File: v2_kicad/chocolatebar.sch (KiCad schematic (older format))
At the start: 155 parts, among them J1 Conn_01x04, SW1 SW_Push, U1 ATmega32U4-AU, Y1 Crystal_GND24_Small

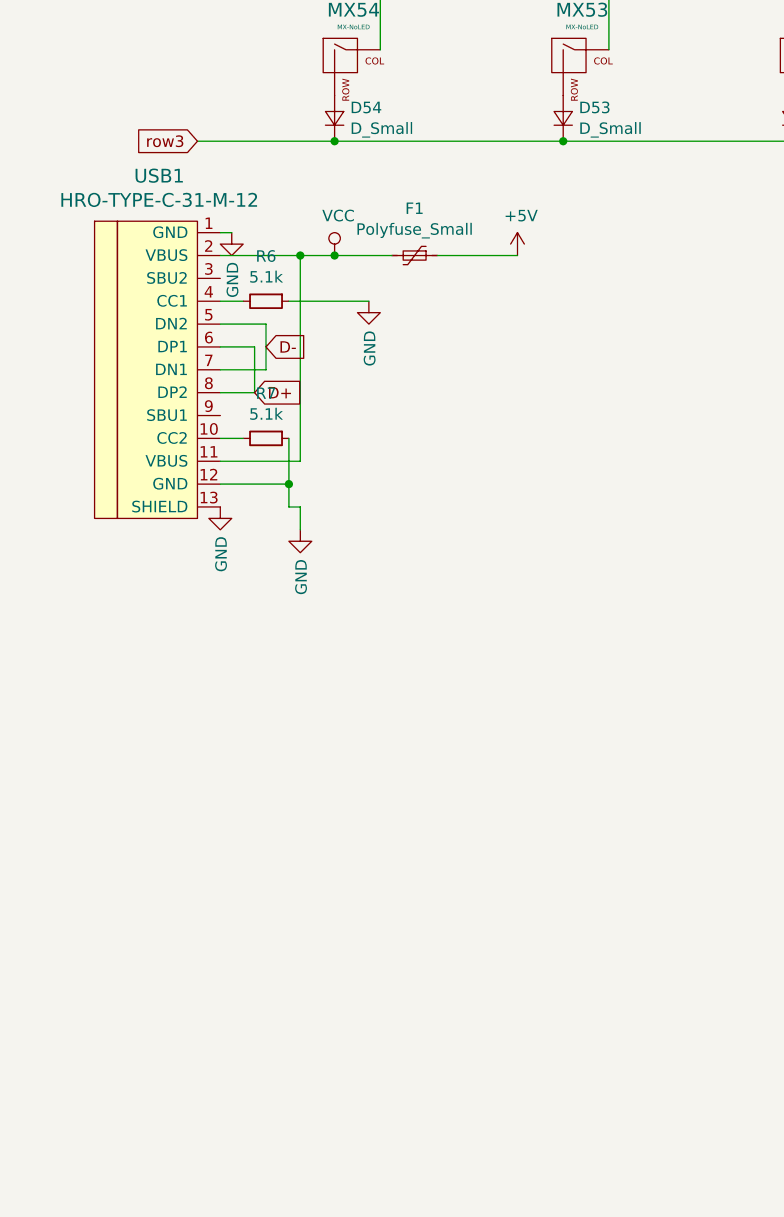
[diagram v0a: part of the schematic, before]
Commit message: V2 update
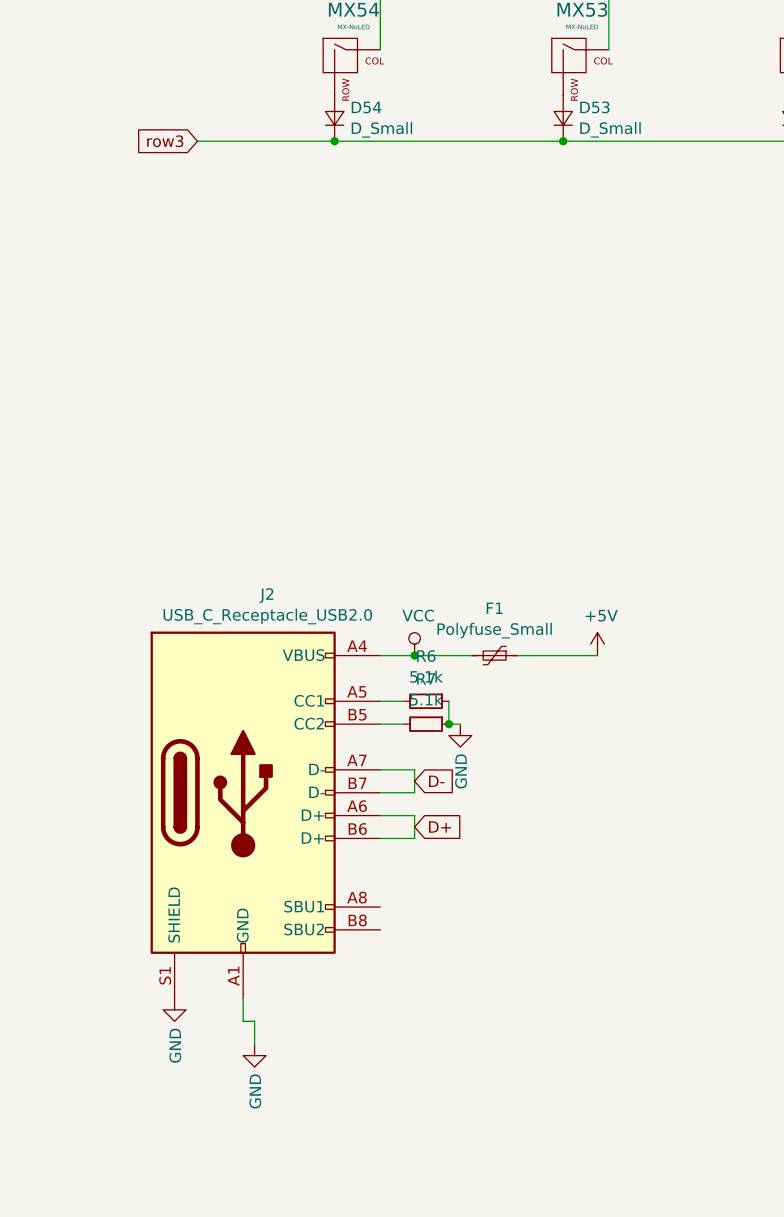
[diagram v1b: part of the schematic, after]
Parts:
- removed USB1: HRO-TYPE-C-31-M-12, Type-C:HRO-TYPE-C-31-M-12-HandSoldering, symbol Type-C:HRO-TYPE-C-31-M-12
- added J2: USB_C_Receptacle_USB2.0, Modified Footprints:USB_C_Receptacle_HRO_TYPE-C-31-M-12, symbol Connector:USB_C_Receptacle_USB2.0
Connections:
- net D+: now also J2.A6 (D+), J2.B6 (D+)
- net D-: now also J2.A7 (D-), J2.B7 (D-)
- net GND: now also J2.A1 (GND), J2.A12 (GND), J2.B1 (GND), J2.B12 (GND), J2.S1 (SHIELD)
- net VCC: now also J2.A4 (VBUS), J2.A9 (VBUS), J2.B4 (VBUS), J2.B9 (VBUS)
- net at R7.2: now also J2.B5 (CC2)
- net at R6.2: now also J2.A5 (CC1)
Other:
- moved on the sheet: F1, R6, R7
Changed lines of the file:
@@
 L Device:Polyfuse_Small F1
 U 1 1 5F2624EF
-P 1950 4900
-F 0 "F1" V 1745 4900 50  0000 C CNN
-F 1 "Polyfuse_Small" V 1836 4900 50  0000 C CNN
-F 2 "Fuse:Fuse_1206_3216Metric" H 2000 4700 50  0001 L CNN
-F 3 "~" H 1950 4900 50  0001 C CNN
-	1    1950 4900
+P 2300 6650
+F 0 "F1" V 2095 6650 50  0000 C CNN
+F 1 "Polyfuse_Small" V 2186 6650 50  0000 C CNN
+F 2 "Fuse:Fuse_1206_3216Metric" H 2350 6450 50  0001 L CNN
+F 3 "~" H 2300 6650 50  0001 C CNN
+	1    2300 6650
 	0    1    1    0
 $EndComp
@@
 L power:+5V #PWR011
 U 1 1 5F26C945
-P 2400 4900
-F 0 "#PWR011" H 2400 4750 50  0001 C CNN
-F 1 "+5V" H 2415 5073 50  0000 C CNN
-F 2 "" H 2400 4900 50  0001 C CNN
-F 3 "" H 2400 4900 50  0001 C CNN
-	1    2400 4900
+P 2750 6650
+F 0 "#PWR011" H 2750 6500 50  0001 C CNN
+F 1 "+5V" H 2765 6823 50  0000 C CNN
+F 2 "" H 2750 6650 50  0001 C CNN
+F 3 "" H 2750 6650 50  0001 C CNN
+	1    2750 6650
 	1    0    0    -1
 $EndComp
@@
 L power:VCC #PWR02
 U 1 1 5F26E1DC
-P 1600 4900
-F 0 "#PWR02" H 1600 4750 50  0001 C CNN
-F 1 "VCC" H 1617 5073 50  0000 C CNN
-F 2 "" H 1600 4900 50  0001 C CNN
-F 3 "" H 1600 4900 50  0001 C CNN
-	1    1600 4900
-	1    0    0    -1
-$EndComp
-Connection ~ 1600 4900
-Wire Wire Line
-	1600 4900 1850 4900
-Wire Wire Line
-	2050 4900 2400 4900
-Text GLabel 1250 5500 2    50   Input ~ 0
+P 1950 6650
+F 0 "#PWR02" H 1950 6500 50  0001 C CNN
+F 1 "VCC" H 1967 6823 50  0000 C CNN
+F 2 "" H 1950 6650 50  0001 C CNN
+F 3 "" H 1950 6650 50  0001 C CNN
+	1    1950 6650
+	1    0    0    -1
+$EndComp
+Connection ~ 1950 6650
+Wire Wire Line
+	1950 6650 2200 6650
+Wire Wire Line
+	2400 6650 2750 6650
+Text GLabel 1950 7400 2    50   Input ~ 0
 D+
-Text GLabel 1300 5300 2    50   Input ~ 0
+Text GLabel 1950 7200 2    50   Input ~ 0
 D-
-$Comp
-L power:GND #PWR01
-U 1 1 5F2AB771
-P 1150 4800
-F 0 "#PWR01" H 1150 4550 50  0001 C CNN
-F 1 "GND" V 1155 4672 50  0000 R CNN
-F 2 "" H 1150 4800 50  0001 C CNN
-F 3 "" H 1150 4800 50  0001 C CNN
-	1    1150 4800
-	1    0    0    -1
-$EndComp
-$Comp
-L Type-C:HRO-TYPE-C-31-M-12 USB1
-U 1 1 5F08F542
-P 1000 5350
-F 0 "USB1" H 833 6147 60  0000 C CNN
-F 1 "HRO-TYPE-C-31-M-12" H 833 6041 60  0000 C CNN
-F 2 "Type-C:HRO-TYPE-C-31-M-12-HandSoldering" H 1000 5350 60  0001 C CNN
-F 3 "" H 1000 5350 60  0001 C CNN
-	1    1000 5350
-	1    0    0    -1
-$EndComp
 Text GLabel 11400 5350 0    50   Input ~ 0
 2812b_data
 Wire Wire Line
-	1100 4900 1450 4900
-Wire Wire Line
-	1100 4800 1150 4800
-Wire Wire Line
-	1100 5800 1450 5800
-Wire Wire Line
-	1450 5800 1450 4900
-Connection ~ 1450 4900
-Wire Wire Line
-	1450 4900 1600 4900
-Wire Wire Line
-	1100 5300 1250 5300
-Wire Wire Line
-	1250 5300 1250 5500
-Wire Wire Line
-	1250 5500 1100 5500
-Wire Wire Line
-	1100 5400 1300 5400
-Wire Wire Line
-	1300 5400 1300 5200
-Wire Wire Line
-	1300 5200 1100 5200
+	1800 6650 1950 6650
 $Comp
 L Device:R_Small R6
 U 1 1 5F5F0D7E
-P 1300 5100
-F 0 "R6" V 1104 5100 50  0000 C CNN
-F 1 "5.1k" V 1195 5100 50  0000 C CNN
-F 2 "Resistor_SMD:R_0805_2012Metric" H 1300 5100 50  0001 C CNN
-F 3 "~" H 1300 5100 50  0001 C CNN
-	1    1300 5100
+P 2000 6850
+F 0 "R6" V 1804 6850 50  0000 C CNN
+F 1 "5.1k" V 1895 6850 50  0000 C CNN
+F 2 "Resistor_SMD:R_0805_2012Metric" H 2000 6850 50  0001 C CNN
+F 3 "~" H 2000 6850 50  0001 C CNN
+	1    2000 6850
 	0    1    1    0
 $EndComp
@@
 L Device:R_Small R7
 U 1 1 5F5FC7F5
-P 1300 5700
-F 0 "R7" V 1104 5700 50  0000 C CNN
-F 1 "5.1k" V 1195 5700 50  0000 C CNN
-F 2 "Resistor_SMD:R_0805_2012Metric" H 1300 5700 50  0001 C CNN
-F 3 "~" H 1300 5700 50  0001 C CNN
-	1    1300 5700
+P 2000 6950
+F 0 "R7" V 1804 6950 50  0000 C CNN
+F 1 "5.1k" V 1895 6950 50  0000 C CNN
+F 2 "Resistor_SMD:R_0805_2012Metric" H 2000 6950 50  0001 C CNN
+F 3 "~" H 2000 6950 50  0001 C CNN
+	1    2000 6950
 	0    1    1    0
 $EndComp
 Wire Wire Line
-	1200 5700 1100 5700
-Wire Wire Line
-	1200 5100 1100 5100
+	1900 6950 1800 6950
+Wire Wire Line
+	1900 6850 1800 6850
 $Comp
 L power:GND #PWR025
 U 1 1 5F647AA1
-P 1750 5100
-F 0 "#PWR025" H 1750 4850 50  0001 C CNN
-F 1 "GND" V 1755 4972 50  0000 R CNN
-F 2 "" H 1750 5100 50  0001 C CNN
-F 3 "" H 1750 5100 50  0001 C CNN
-	1    1750 5100
+P 2150 6950
+F 0 "#PWR025" H 2150 6700 50  0001 C CNN
+F 1 "GND" V 2155 6822 50  0000 R CNN
+F 2 "" H 2150 6950 50  0001 C CNN
+F 3 "" H 2150 6950 50  0001 C CNN
+	1    2150 6950
 	1    0    0    -1
 $EndComp
@@
 L power:GND #PWR024
 U 1 1 5F68571B
-P 1450 6100
-F 0 "#PWR024" H 1450 5850 50  0001 C CNN
-F 1 "GND" V 1455 5972 50  0000 R CNN
-F 2 "" H 1450 6100 50  0001 C CNN
-F 3 "" H 1450 6100 50  0001 C CNN
-	1    1450 6100
-	1    0    0    -1
-$EndComp
-Wire Wire Line
-	1450 6000 1450 6100
-Wire Wire Line
-	1450 6000 1400 6000
-Wire Wire Line
-	1400 5700 1400 5900
-Wire Wire Line
-	1400 5100 1750 5100
-Wire Wire Line
-	1100 5900 1400 5900
-Connection ~ 1400 5900
-Wire Wire Line
-	1400 5900 1400 6000
+P 1250 8350
+F 0 "#PWR024" H 1250 8100 50  0001 C CNN
+F 1 "GND" V 1255 8222 50  0000 R CNN
+F 2 "" H 1250 8350 50  0001 C CNN
+F 3 "" H 1250 8350 50  0001 C CNN
+	1    1250 8350
+	1    0    0    -1
+$EndComp
+Wire Wire Line
+	1250 8250 1250 8350
+Wire Wire Line
+	1250 8250 1200 8250
+Wire Wire Line
+	1200 8150 1200 8250
 Text GLabel 8150 8050 2    50   Input ~ 0
 col2
@@
 L power:GND #PWR0121
 U 1 1 5F95F16A
-P 1100 6000
-F 0 "#PWR0121" H 1100 5750 50  0001 C CNN
-F 1 "GND" V 1105 5872 50  0000 R CNN
-F 2 "" H 1100 6000 50  0001 C CNN
-F 3 "" H 1100 6000 50  0001 C CNN
-	1    1100 6000
+P 900 8150
+F 0 "#PWR0121" H 900 7900 50  0001 C CNN
+F 1 "GND" V 905 8022 50  0000 R CNN
+F 2 "" H 900 8150 50  0001 C CNN
+F 3 "" H 900 8150 50  0001 C CNN
+	1    900  8150
 	1    0    0    -1
 $EndComp
@@
 Text GLabel 8150 6750 2    50   Input ~ 0
 SDA
+$Comp
+L Connector:USB_C_Receptacle_USB2.0 J2
+U 1 1 60A71C53
+P 1200 7250
+F 0 "J2" H 1307 8117 50  0000 C CNN
+F 1 "USB_C_Receptacle_USB2.0" H 1307 8026 50  0000 C CNN
+F 2 "Modified Footprints:USB_C_Receptacle_HRO_TYPE-C-31-M-12" H 1350 7250 50  0001 C CNN
+F 3 "https://www.usb.org/sites/default/files/documents/usb_type-c.zip" H 1350 7250 50  0001 C CNN
+	1    1200 7250
+	1    0    0    -1
+$EndComp
+Wire Wire Line
+	2150 6950 2100 6950
+Wire Wire Line
+	2100 6950 2100 6850
+Connection ~ 2100 6950
+Wire Wire Line
+	1800 7250 1950 7250
+Wire Wire Line
+	1950 7250 1950 7150
+Wire Wire Line
+	1950 7150 1800 7150
+Wire Wire Line
+	1800 7350 1950 7350
+Wire Wire Line
+	1950 7350 1950 7450
+Wire Wire Line
+	1950 7450 1800 7450
 $EndSCHEMATC
